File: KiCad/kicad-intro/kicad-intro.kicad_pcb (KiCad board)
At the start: 2 copper layers, 9 parts, among them U1 D168K

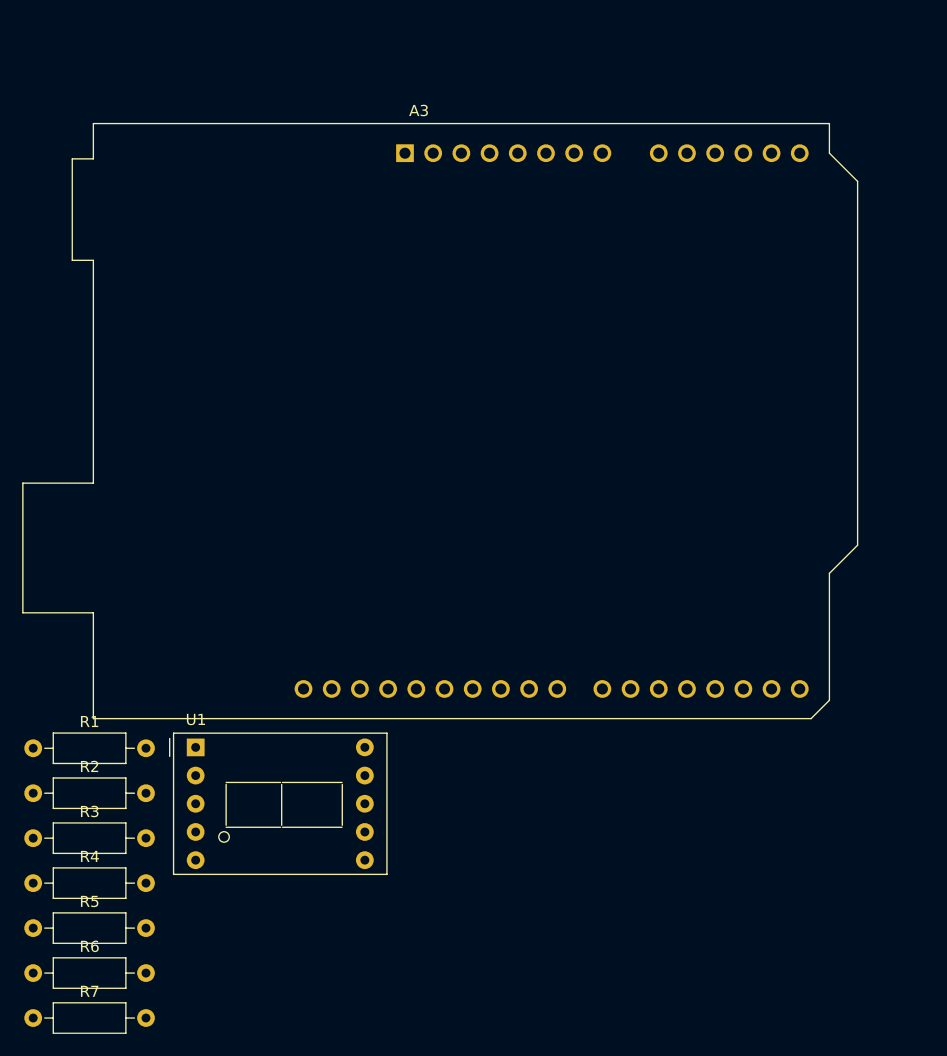
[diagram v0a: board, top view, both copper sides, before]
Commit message: trying to resolve conflicts...
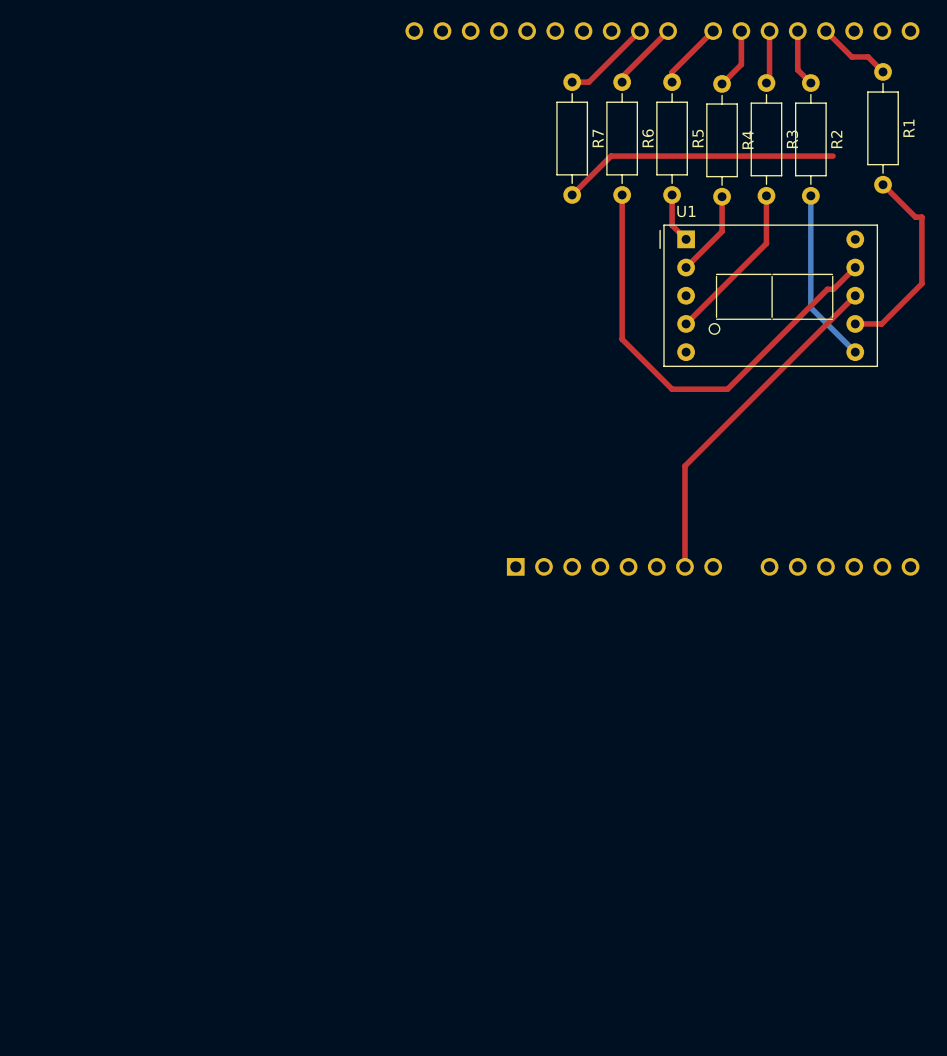
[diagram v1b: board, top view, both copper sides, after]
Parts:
- A3: moved to B.Cu
- moved R1 97.8 mm to (174.5, 67.4), turned to -90 degrees
- moved R7 97.3 mm to (146.5, 68.3), turned to -90 degrees
- moved R6 96.2 mm to (151.0, 68.3), turned to -90 degrees
- moved R5 95.5 mm to (155.5, 68.3), turned to -90 degrees
- moved R4 95.0 mm to (160.0, 68.5), turned to -90 degrees
- moved R2 94.9 mm to (168.0, 68.4), turned to -90 degrees
- moved R3 94.8 mm to (164.0, 68.4), turned to -90 degrees
- moved U1 63.6 mm to (156.8, 82.5)
- moved A3 38.6 mm to (141.4, 112.0)
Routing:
- net Net-(U1-F): track 0.00 -> 40.4 mm
- net Net-(A3-GND-Pad7): track 0.00 -> 30.8 mm
- net /7-seg-G: track 0.00 -> 24.9 mm
- net Net-(U1-A): track 0.00 -> 18.2 mm
- net Net-(U1-B): track 0.00 -> 15.7 mm
- net Net-(U1-C): track 0.00 -> 14.5 mm
- net /D9: track 0.00 -> 8.01 mm
- net Net-(U1-D): track 0.00 -> 7.72 mm
- net Net-(A3-D3): track 0.00 -> 6.66 mm
- net Net-(A3-D8): track 0.00 -> 6.31 mm
- net Net-(A3-D7): track 0.00 -> 6.13 mm
- net Net-(A3-D6): track 0.00 -> 5.48 mm
- net Net-(A3-D4): track 0.00 -> 5.17 mm
- net Net-(A3-D5): track 0.00 -> 4.80 mm
- net Net-(U1-E): track 0.00 -> 4.52 mm
